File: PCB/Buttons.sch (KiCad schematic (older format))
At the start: 15 parts

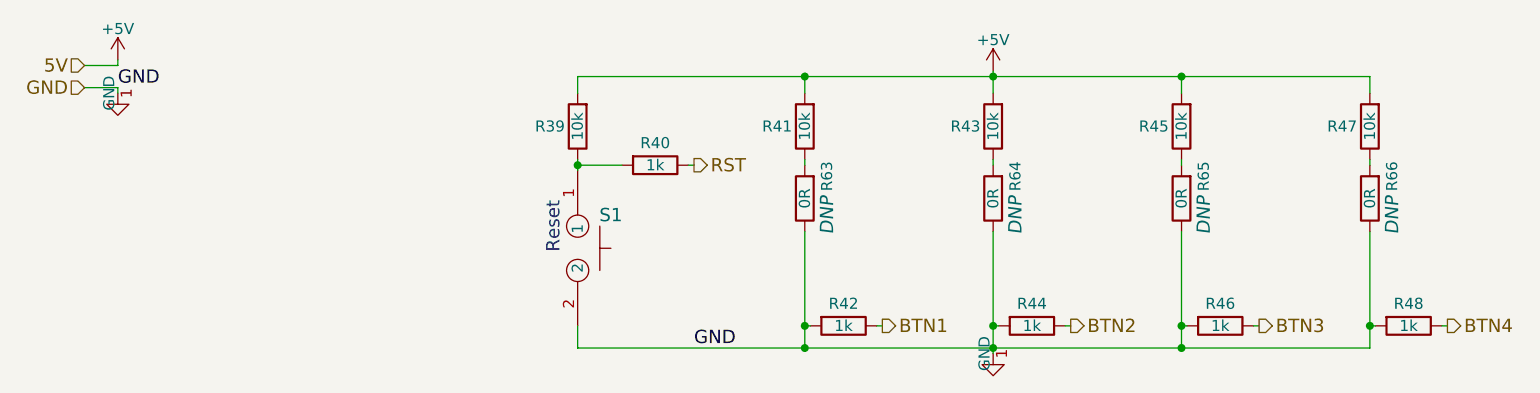
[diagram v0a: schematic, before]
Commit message: ./
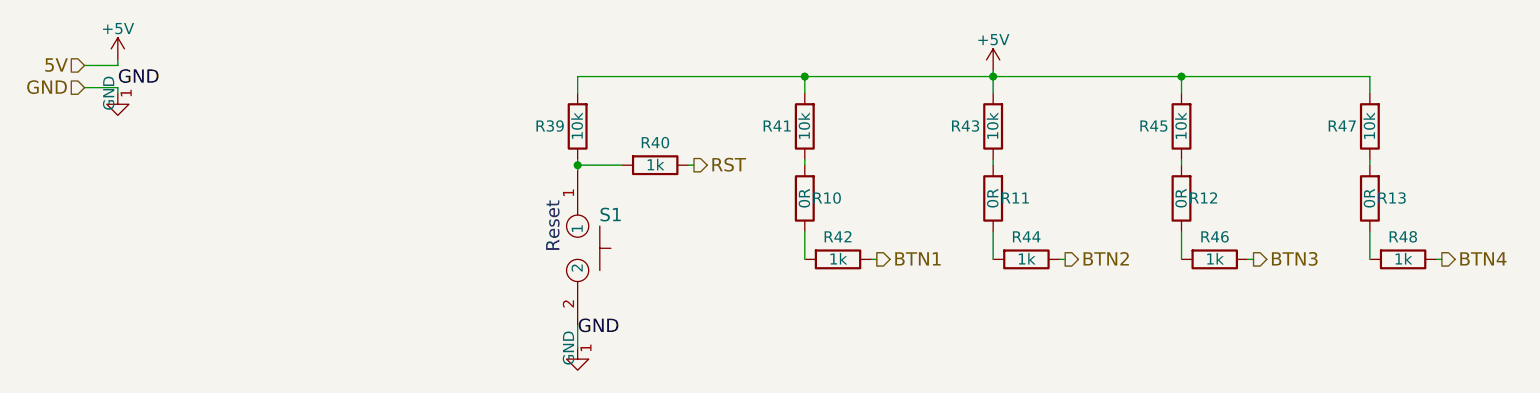
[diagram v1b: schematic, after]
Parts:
- removed R63, R64, R65, R66: 0R, Resistor_THT:R_Axial_DIN0207_L6.3mm_D2.5mm_P2.54mm_Vertical, symbol R
- added R10, R11, R12, R13: 0R, Resistor_THT:R_Axial_DIN0204_L3.6mm_D1.6mm_P2.54mm_Vertical, symbol R
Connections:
- net GND: no longer R42.2, R44.2, R46.2, R48.2
- net at R41.1: now also R10.2
- net at R43.1: now also R11.2
- net at R45.1: now also R12.2
- net at R47.1: now also R13.2
- new net: R10.1, R42.2
- new net: R11.1, R44.2
- new net: R12.1, R46.2
- new net: R13.1, R48.2
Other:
- moved on the sheet: R42, R44, R46, R48
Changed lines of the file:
@@
 L R R42
 U 1 1 5A1EF484
-P 4700 4100
-F 0 "R42" V 4600 4100 50  0000 C CNN
-F 1 "1k" V 4700 4100 50  0000 C CNN
-F 2 "Resistors_SMD:R_0603_HandSoldering" V 4630 4100 50  0001 C CNN
-F 3 "" H 4700 4100 50  0001 C CNN
-	1    4700 4100
+P 4675 3800
+F 0 "R42" V 4575 3800 50  0000 C CNN
+F 1 "1k" V 4675 3800 50  0000 C CNN
+F 2 "Resistors_SMD:R_0603_HandSoldering" V 4605 3800 50  0001 C CNN
+F 3 "" H 4675 3800 50  0001 C CNN
+	1    4675 3800
 	0    1    1    0
 $EndComp
@@
 L R R44
 U 1 1 5A1EF4A7
-P 5550 4100
-F 0 "R44" V 5450 4100 50  0000 C CNN
-F 1 "1k" V 5550 4100 50  0000 C CNN
-F 2 "Resistors_SMD:R_0603_HandSoldering" V 5480 4100 50  0001 C CNN
-F 3 "" H 5550 4100 50  0001 C CNN
-	1    5550 4100
+P 5525 3800
+F 0 "R44" V 5425 3800 50  0000 C CNN
+F 1 "1k" V 5525 3800 50  0000 C CNN
+F 2 "Resistors_SMD:R_0603_HandSoldering" V 5455 3800 50  0001 C CNN
+F 3 "" H 5525 3800 50  0001 C CNN
+	1    5525 3800
 	0    1    1    0
 $EndComp
@@
 L R R46
 U 1 1 5A1EF4C9
-P 6400 4100
-F 0 "R46" V 6300 4100 50  0000 C CNN
-F 1 "1k" V 6400 4100 50  0000 C CNN
-F 2 "Resistors_SMD:R_0603_HandSoldering" V 6330 4100 50  0001 C CNN
-F 3 "" H 6400 4100 50  0001 C CNN
-	1    6400 4100
+P 6375 3800
+F 0 "R46" V 6275 3800 50  0000 C CNN
+F 1 "1k" V 6375 3800 50  0000 C CNN
+F 2 "Resistors_SMD:R_0603_HandSoldering" V 6305 3800 50  0001 C CNN
+F 3 "" H 6375 3800 50  0001 C CNN
+	1    6375 3800
 	0    1    1    0
 $EndComp
@@
 L R R48
 U 1 1 5A1EF4EB
-P 7250 4100
-F 0 "R48" V 7150 4100 50  0000 C CNN
-F 1 "1k" V 7250 4100 50  0000 C CNN
-F 2 "Resistors_SMD:R_0603_HandSoldering" V 7180 4100 50  0001 C CNN
-F 3 "" H 7250 4100 50  0001 C CNN
-	1    7250 4100
+P 7225 3800
+F 0 "R48" V 7125 3800 50  0000 C CNN
+F 1 "1k" V 7225 3800 50  0000 C CNN
+F 2 "Resistors_SMD:R_0603_HandSoldering" V 7155 3800 50  0001 C CNN
+F 3 "" H 7225 3800 50  0001 C CNN
+	1    7225 3800
 	0    1    1    0
 $EndComp
 Text HLabel 4025 3375 2    60   Output ~ 0
 RST
-Text HLabel 4875 4100 2    60   Output ~ 0
+Text HLabel 4850 3800 2    60   Output ~ 0
 BTN1
-Text HLabel 5725 4100 2    60   Output ~ 0
+Text HLabel 5700 3800 2    60   Output ~ 0
 BTN2
-Text HLabel 6575 4100 2    60   Output ~ 0
+Text HLabel 6550 3800 2    60   Output ~ 0
 BTN3
-Text HLabel 7425 4100 2    60   Output ~ 0
+Text HLabel 7400 3800 2    60   Output ~ 0
 BTN4
 Text HLabel 1275 3025 0    60   Input ~ 0
 GND
 $Comp
-L GND-RESCUE-Tardis #PWR062
+L GND-RESCUE-Tardis #PWR63
 U 1 1 5A341B2F
 P 1425 3050
-F 0 "#PWR062" H 1425 2800 50  0001 C CNN
+F 0 "#PWR63" H 1425 2800 50  0001 C CNN
 F 1 "GND" H 1425 2900 50  0001 C CNN
 F 2 "" H 1425 3050 50  0001 C CNN
@@
 	1425 3025 1425 3050
 $Comp
-L +5V #PWR063
+L +5V #PWR62
 U 1 1 5A341B37
 P 1425 2900
-F 0 "#PWR063" H 1425 2750 50  0001 C CNN
+F 0 "#PWR62" H 1425 2750 50  0001 C CNN
 F 1 "+5V" H 1425 3040 50  0000 C CNN
 F 2 "" H 1425 2900 50  0001 C CNN
@@
 	3500 3350 3500 3400
 $Comp
-L +5V #PWR064
+L +5V #PWR65
 U 1 1 5A342622
 P 5375 2950
-F 0 "#PWR064" H 5375 2800 50  0001 C CNN
+F 0 "#PWR65" H 5375 2800 50  0001 C CNN
 F 1 "+5V" H 5375 3090 50  0000 C CNN
 F 2 "" H 5375 2950 50  0001 C CNN
@@
 $EndComp
 $Comp
-L GND-RESCUE-Tardis #PWR065
+L GND-RESCUE-Tardis #PWR64
 U 1 1 5A34265A
-P 5375 4225
-F 0 "#PWR065" H 5375 3975 50  0001 C CNN
-F 1 "GND" H 5375 4075 50  0001 C CNN
-F 2 "" H 5375 4225 50  0001 C CNN
-F 3 "" H 5375 4225 50  0001 C CNN
-	1    5375 4225
-	1    0    0    -1
-$EndComp
-Wire Wire Line
-	4525 3350 4525 3375
-Wire Wire Line
-	4525 3675 4525 4200
-Wire Wire Line
-	4525 4100 4550 4100
-Wire Wire Line
-	4850 4100 4875 4100
-Wire Wire Line
-	5700 4100 5725 4100
-Wire Wire Line
-	5400 4100 5375 4100
-Wire Wire Line
-	5375 3675 5375 4225
-Wire Wire Line
-	6225 4200 6225 3675
-Wire Wire Line
-	6225 4100 6250 4100
-Wire Wire Line
-	6550 4100 6575 4100
-Wire Wire Line
-	6225 3375 6225 3350
-Wire Wire Line
-	7100 4100 7075 4100
-Wire Wire Line
-	7075 4200 7075 3675
-Wire Wire Line
-	7425 4100 7400 4100
-Wire Wire Line
-	7075 3375 7075 3350
+P 3500 4200
+F 0 "#PWR64" H 3500 3950 50  0001 C CNN
+F 1 "GND" H 3500 4050 50  0001 C CNN
+F 2 "" H 3500 4200 50  0001 C CNN
+F 3 "" H 3500 4200 50  0001 C CNN
+	1    3500 4200
+	1    0    0    -1
+$EndComp
+Wire Wire Line
+	4825 3800 4850 3800
+Wire Wire Line
+	5675 3800 5700 3800
+Wire Wire Line
+	6525 3800 6550 3800
+Wire Wire Line
+	7400 3800 7375 3800
 Wire Wire Line
 	3500 3050 3500 2975
@@
 Connection ~ 4525 2975
 Wire Wire Line
-	3500 4200 7075 4200
-Connection ~ 7075 4100
-Connection ~ 5375 4200
-Connection ~ 5375 4100
-Connection ~ 4525 4200
-Connection ~ 4525 4100
-Connection ~ 6225 4200
-Connection ~ 6225 4100
-Wire Wire Line
-	5375 3350 5375 3375
-Wire Wire Line
 	3700 3375 3500 3375
 Connection ~ 3500 3375
-Text Label 4025 4200 0    60   ~ 0
+Text Label 3500 4150 0    60   ~ 0
 GND
 Text Label 1425 3025 0    60   ~ 0
 GND
-$Comp
-L R R63
-U 1 1 5A4F3BCE
-P 4525 3525
-F 0 "R63" V 4425 3425 50  0000 C CNN
-F 1 "0R" V 4525 3525 50  0000 C CNN
-F 2 "Resistor_THT:R_Axial_DIN0207_L6.3mm_D2.5mm_P2.54mm_Vertical" V 4455 3525 50  0001 C CNN
-F 3 "" H 4525 3525 50  0001 C CNN
-F 4 "Jumper" V 4425 3600 39  0001 C CNN "%"
-F 5 "DNP" V 4425 3600 60  0000 C CIN "DNP"
-F 6 "A105988CT-ND" V 4525 3525 60  0001 C CNN "Digikey"
-	1    4525 3525
-	-1   0    0    1
-$EndComp
 $Comp
 L mom_button S1
@@
 $EndComp
 $Comp
-L R R64
-U 1 1 5A4F426C
+L R R10
+U 1 1 5A59E758
+P 4525 3525
+F 0 "R10" H 4425 3525 50  0000 C CNN
+F 1 "0R" V 4525 3525 50  0000 C CNN
+F 2 "Resistor_THT:R_Axial_DIN0204_L3.6mm_D1.6mm_P2.54mm_Vertical" V 4455 3525 50  0001 C CNN
+F 3 "" H 4525 3525 50  0001 C CNN
+	1    4525 3525
+	-1   0    0    1
+$EndComp
+Wire Wire Line
+	4525 3350 4525 3375
+Wire Wire Line
+	4525 3675 4525 3800
+Wire Wire Line
+	5375 3350 5375 3375
+Wire Wire Line
+	5375 3675 5375 3800
+Wire Wire Line
+	6225 3350 6225 3375
+Wire Wire Line
+	6225 3675 6225 3800
+Wire Wire Line
+	7075 3675 7075 3800
+Wire Wire Line
+	7075 3375 7075 3350
+$Comp
+L R R11
+U 1 1 5A5A04BC
 P 5375 3525
-F 0 "R64" V 5275 3425 50  0000 C CNN
+F 0 "R11" H 5275 3525 50  0000 C CNN
 F 1 "0R" V 5375 3525 50  0000 C CNN
-F 2 "Resistor_THT:R_Axial_DIN0207_L6.3mm_D2.5mm_P2.54mm_Vertical" V 5305 3525 50  0001 C CNN
+F 2 "Resistor_THT:R_Axial_DIN0204_L3.6mm_D1.6mm_P2.54mm_Vertical" V 5305 3525 50  0001 C CNN
 F 3 "" H 5375 3525 50  0001 C CNN
-F 4 "Jumper" V 5275 3600 39  0001 C CNN "%"
-F 5 "DNP" V 5275 3600 60  0000 C CIN "DNP"
-F 6 "A105988CT-ND" V 5375 3525 60  0001 C CNN "Digikey"
 	1    5375 3525
 	-1   0    0    1
 $EndComp
 $Comp
-L R R65
-U 1 1 5A4F42ED
+L R R12
+U 1 1 5A5A0523
 P 6225 3525
-F 0 "R65" V 6125 3425 50  0000 C CNN
+F 0 "R12" H 6125 3525 50  0000 C CNN
 F 1 "0R" V 6225 3525 50  0000 C CNN
-F 2 "Resistor_THT:R_Axial_DIN0207_L6.3mm_D2.5mm_P2.54mm_Vertical" V 6155 3525 50  0001 C CNN
+F 2 "Resistor_THT:R_Axial_DIN0204_L3.6mm_D1.6mm_P2.54mm_Vertical" V 6155 3525 50  0001 C CNN
 F 3 "" H 6225 3525 50  0001 C CNN
-F 4 "Jumper" V 6125 3600 39  0001 C CNN "%"
-F 5 "DNP" V 6125 3600 60  0000 C CIN "DNP"
-F 6 "A105988CT-ND" V 6225 3525 60  0001 C CNN "Digikey"
 	1    6225 3525
 	-1   0    0    1
 $EndComp
 $Comp
-L R R66
-U 1 1 5A4F4359
+L R R13
+U 1 1 5A5A057B
 P 7075 3525
-F 0 "R66" V 6975 3425 50  0000 C CNN
+F 0 "R13" H 6975 3525 50  0000 C CNN
 F 1 "0R" V 7075 3525 50  0000 C CNN
-F 2 "Resistor_THT:R_Axial_DIN0207_L6.3mm_D2.5mm_P2.54mm_Vertical" V 7005 3525 50  0001 C CNN
+F 2 "Resistor_THT:R_Axial_DIN0204_L3.6mm_D1.6mm_P2.54mm_Vertical" V 7005 3525 50  0001 C CNN
 F 3 "" H 7075 3525 50  0001 C CNN
-F 4 "Jumper" V 6975 3600 39  0001 C CNN "%"
-F 5 "DNP" V 6975 3600 60  0000 C CIN "DNP"
-F 6 "A105988CT-ND" V 7075 3525 60  0001 C CNN "Digikey"
 	1    7075 3525
 	-1   0    0    1
